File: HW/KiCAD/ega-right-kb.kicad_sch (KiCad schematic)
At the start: 113 parts, among them SW00 SW_Push, SW01 SW_Push, SW02 SW_Push, SW03 SW_Push, SW04 SW_Push, SW05 SW_Push, SW06 SW_Push, SW07 SW_Push, SW08 SW_Push, SW10 SW_Push, SW11 SW_Push, SW12 SW_Push, SW13 SW_Push, SW14 SW_Push, SW15 SW_Push, SW16 SW_Push, SW17 SW_Push, SW18 SW_Push, SW19 SW_Push, SW20 SW_Push, SW21 SW_Push, SW22 SW_Push, SW23 SW_Push, SW24 SW_Push, SW25 SW_Push, SW26 SW_Push, SW27 SW_Push, SW28 SW_Push, SW29 SW_Push, SW30 SW_Push, SW31 SW_Push, SW32 SW_Push, SW33 SW_Push, SW34 SW_Push, SW35 SW_Push, SW36 SW_Push, SW37 SW_Push, SW38 SW_Push, SW40 SW_Push, SW41 SW_Push, SW42 SW_Push, SW43 SW_Push, SW44 SW_Push, SW45 SW_Push, SW46 SW_Push, SW47 SW_Push, SW48 SW_Push, SW49 SW_Push, SW50 SW_Push, SW51 SW_Push, SW52 SW_Push, SW53 SW_Push, SW54 SW_Push, SW55 SW_Push, SW56 SW_Push, SW57 SW_Push

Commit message: chore: update code structure for improved readability and maintainability
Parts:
- SW00, SW01, SW02, SW03, SW04, SW05, SW06, SW07, SW08, SW10, SW11, SW12, SW13, SW14, SW15, SW16, SW17, SW18, SW19, SW20, SW21, SW22, SW23, SW24, SW25, SW26, SW27, SW28, SW29, SW30, SW31, SW32, SW33, SW34, SW35, SW36, SW37, SW38, SW40, SW41, SW42, SW43, SW44, SW45, SW46, SW47, SW48, SW49, SW50, SW51, SW52, SW53, SW54, SW55, SW56, SW57: footprint KeySwitch:MX-Hotswap-1U -> PCM_Switch_Keyboard_Hotswap_Kailh:SW_Hotswap_Kailh_MX_1.00u

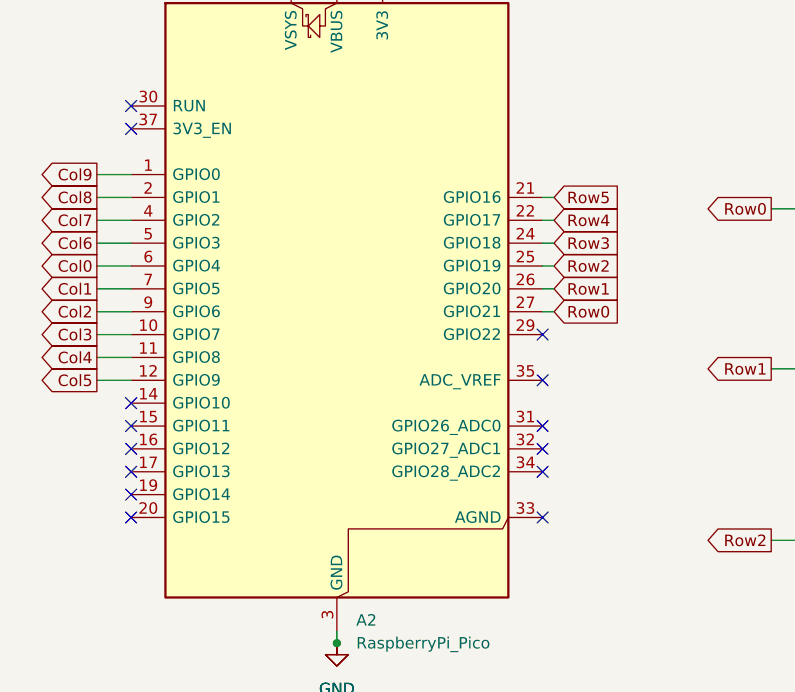
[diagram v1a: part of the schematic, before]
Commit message: chore: メイン基板　の配線まで完成
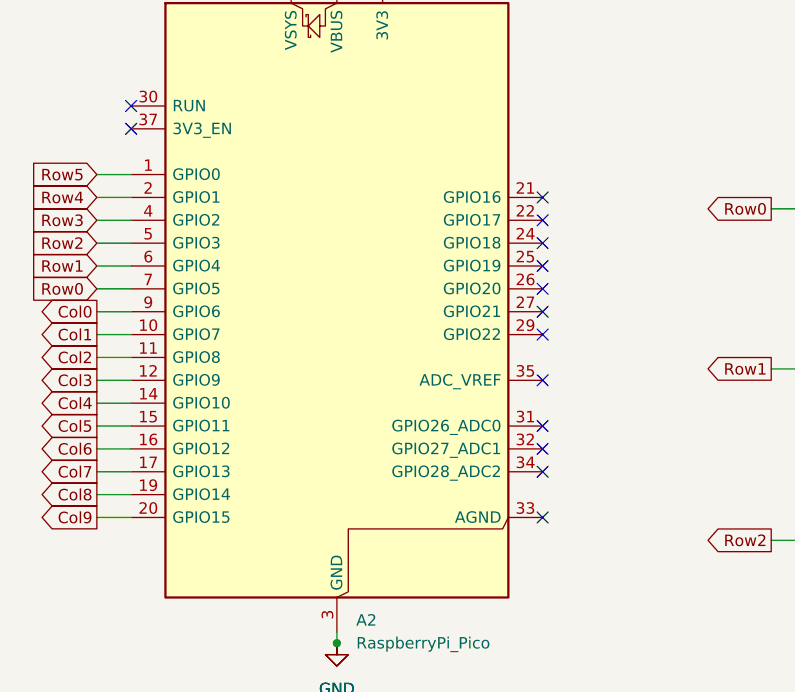
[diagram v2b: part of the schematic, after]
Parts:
- D00, D01, D02, D03, D04, D05, D06, D07, D08, D10, D11, D12, D13, D14, D15, D16, D17, D18, D19, D20, D21, D22, D23, D24, D25, D26, D27, D28, D29, D30, D31, D32, D33, D34, D35, D36, D37, D38, D40, D41, D42, D43, D44, D45, D46, D47, D48, D49, D50, D51, D52, D53, D54, D55, D56, D57: footprint Diode_THT:D_DO-35_SOD27_P7.62mm_Horizontal -> Diode_SMD:D_SOD-123
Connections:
- net Col0: now also A2.9 (GPIO6); no longer A2.6 (GPIO4)
- net Col1: now also A2.10 (GPIO7); no longer A2.7 (GPIO5)
- net Col2: now also A2.11 (GPIO8); no longer A2.9 (GPIO6)
- net Col3: now also A2.12 (GPIO9); no longer A2.10 (GPIO7)
- net Col4: now also A2.14 (GPIO10); no longer A2.11 (GPIO8)
- net Col5: now also A2.15 (GPIO11); no longer A2.12 (GPIO9)
- net Col6: now also A2.16 (GPIO12); no longer A2.5 (GPIO3)
- net Col7: now also A2.17 (GPIO13); no longer A2.4 (GPIO2)
- net Col8: now also A2.19 (GPIO14); no longer A2.2 (GPIO1)
- net Col9: now also A2.20 (GPIO15); no longer A2.1 (GPIO0)
- net Row0: now also A2.7 (GPIO5); no longer A2.27 (GPIO21)
- net Row1: now also A2.6 (GPIO4); no longer A2.26 (GPIO20)
- net Row2: now also A2.5 (GPIO3); no longer A2.25 (GPIO19)
- net Row3: now also A2.4 (GPIO2); no longer A2.24 (GPIO18)
- net Row4: now also A2.2 (GPIO1); no longer A2.22 (GPIO17)
- net Row5: now also A2.1 (GPIO0); no longer A2.21 (GPIO16)
